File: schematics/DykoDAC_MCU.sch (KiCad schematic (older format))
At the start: 43 parts, among them J3 USB_B, J4 OLED, J5 Debug, J6 Encoder_MCU, J7 OLED_MCU, J8 Encoder_IN, J9 OLED_IN, SW1 EC11B152420G, SW2 Button A, SW3 Button B, SW4 The Button, U11 PRTR5V0U2X.215, U13 ATSAMD51J20A-A

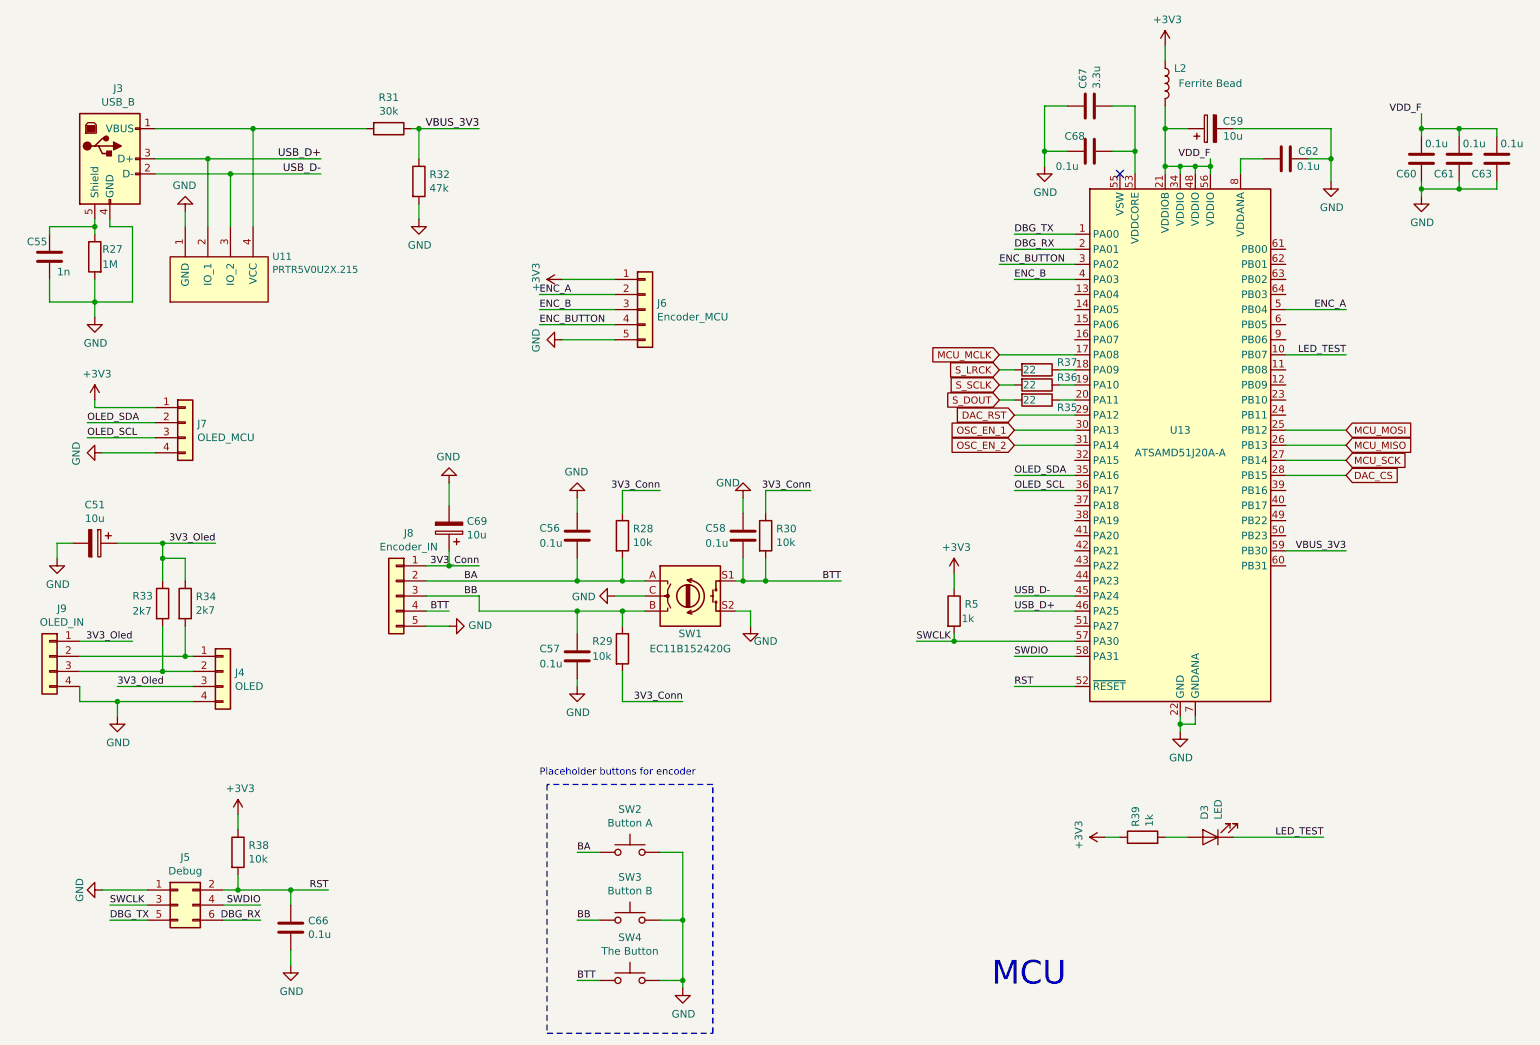
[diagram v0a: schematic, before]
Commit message: minor changes & pdf update
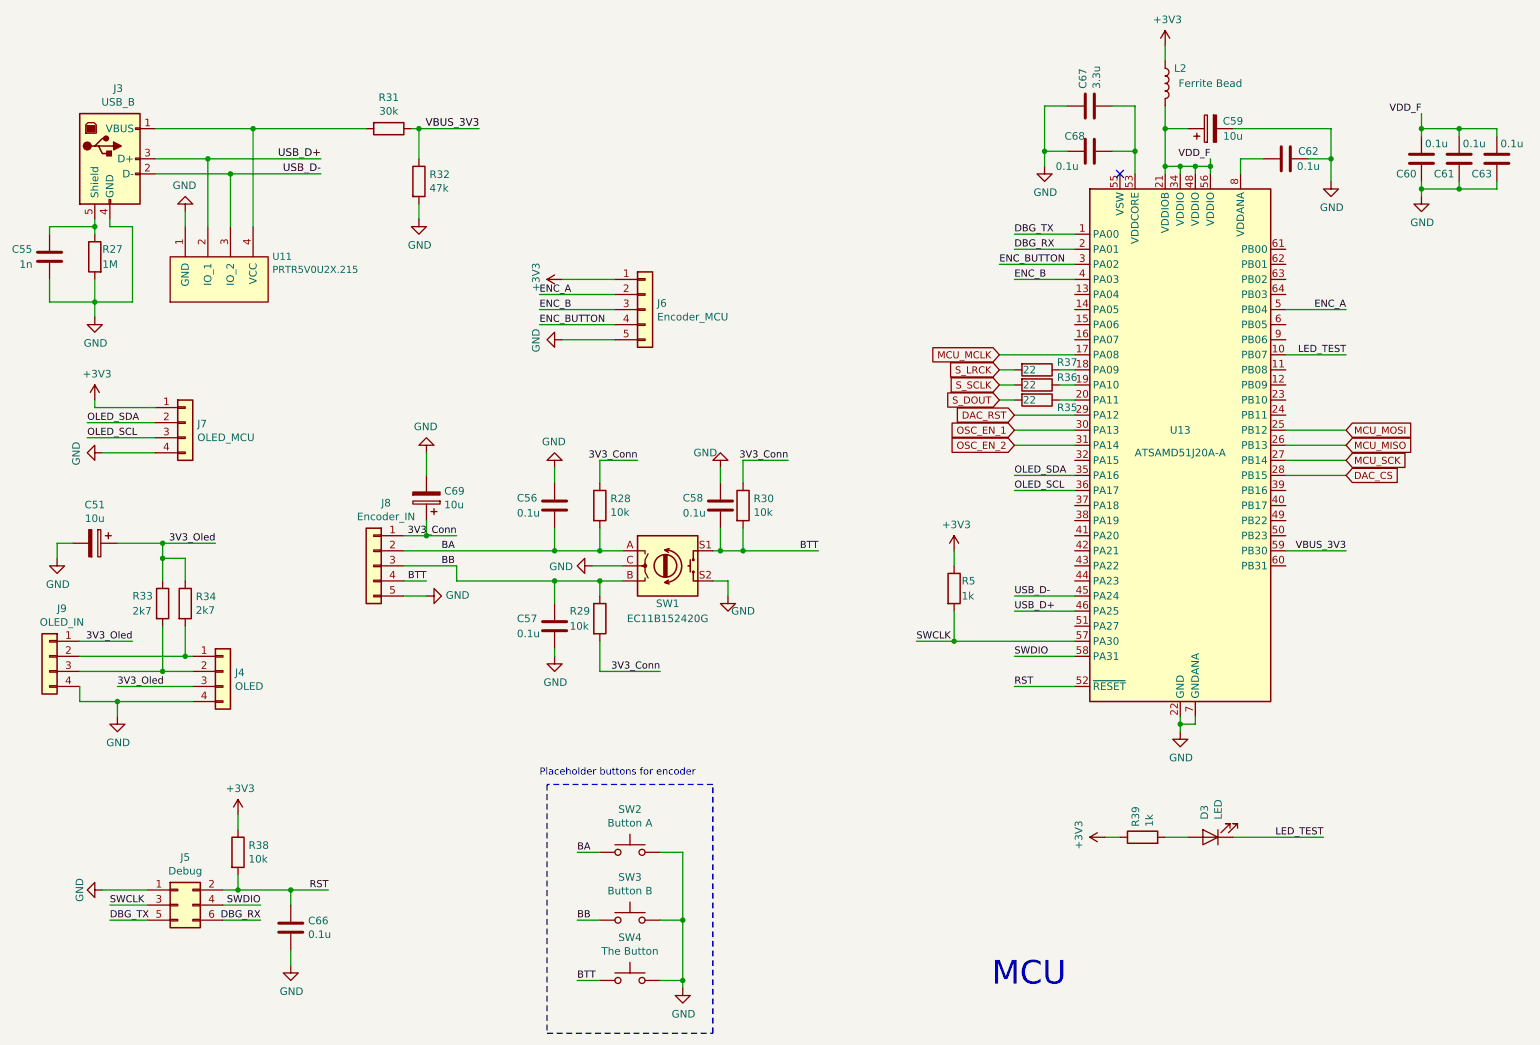
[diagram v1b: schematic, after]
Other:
- moved on the sheet: C56, C57, C58, C69, J8, R28, R29, R30, R5, SW1
